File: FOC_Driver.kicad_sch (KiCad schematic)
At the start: 0 parts

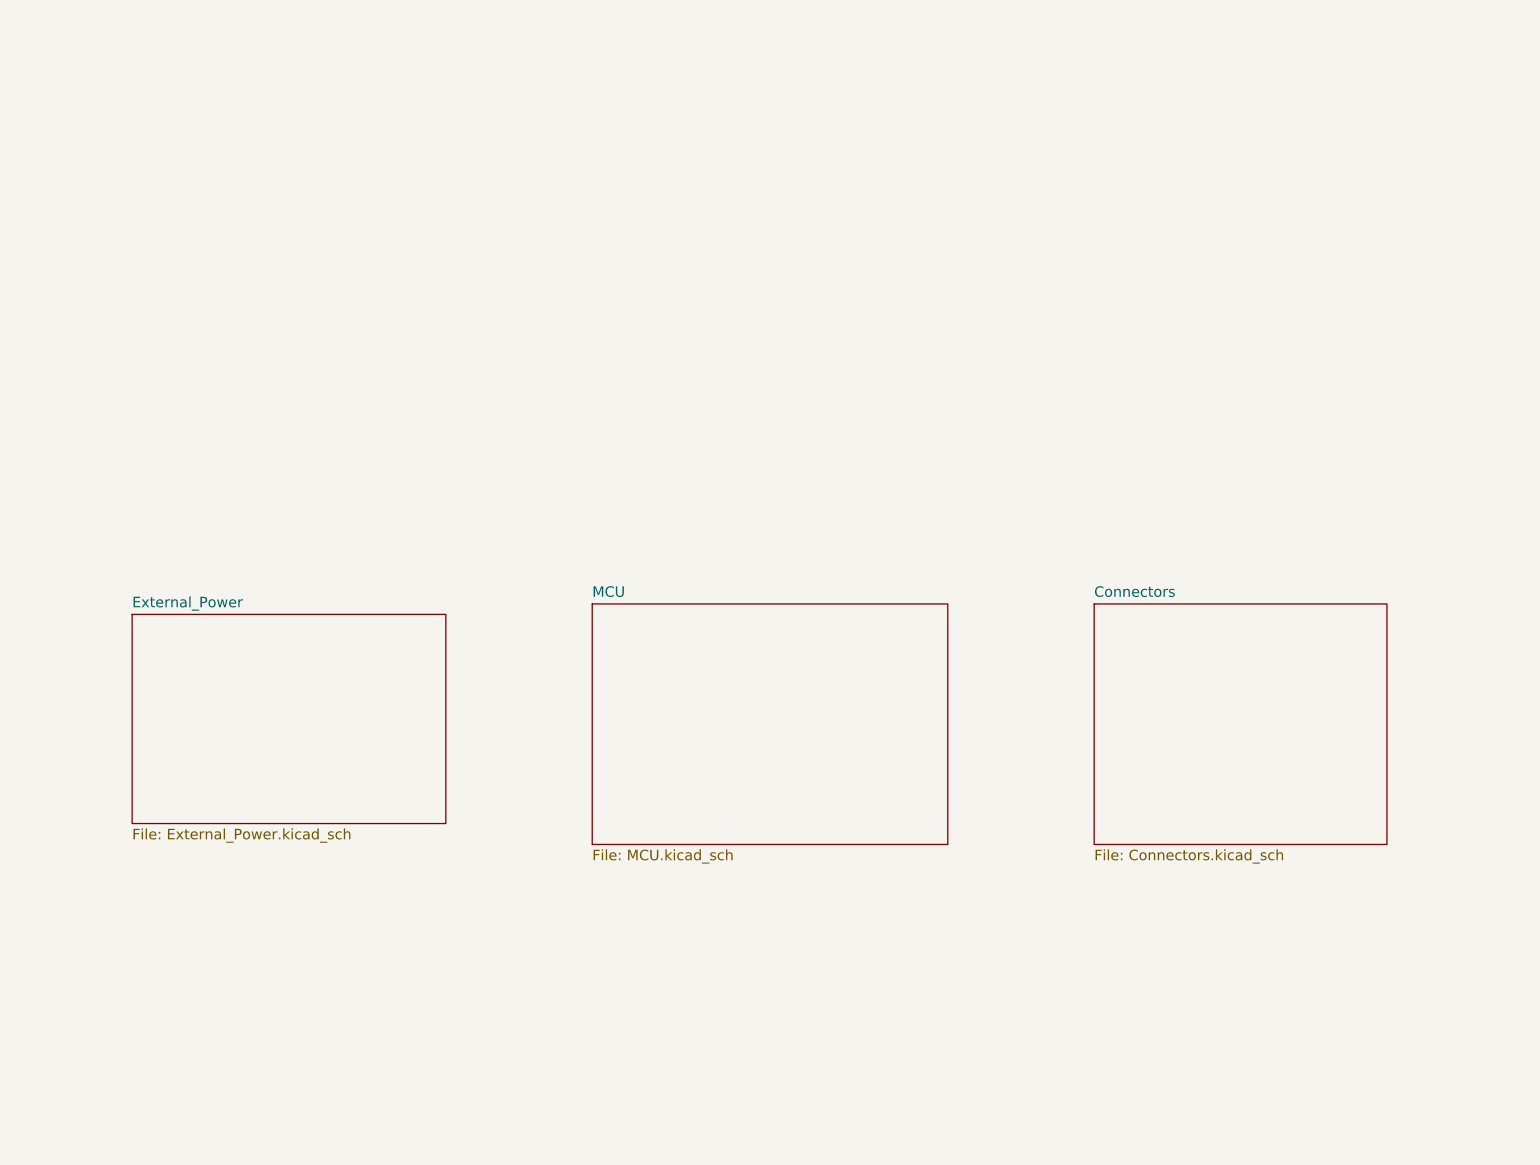
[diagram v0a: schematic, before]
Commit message: Wip
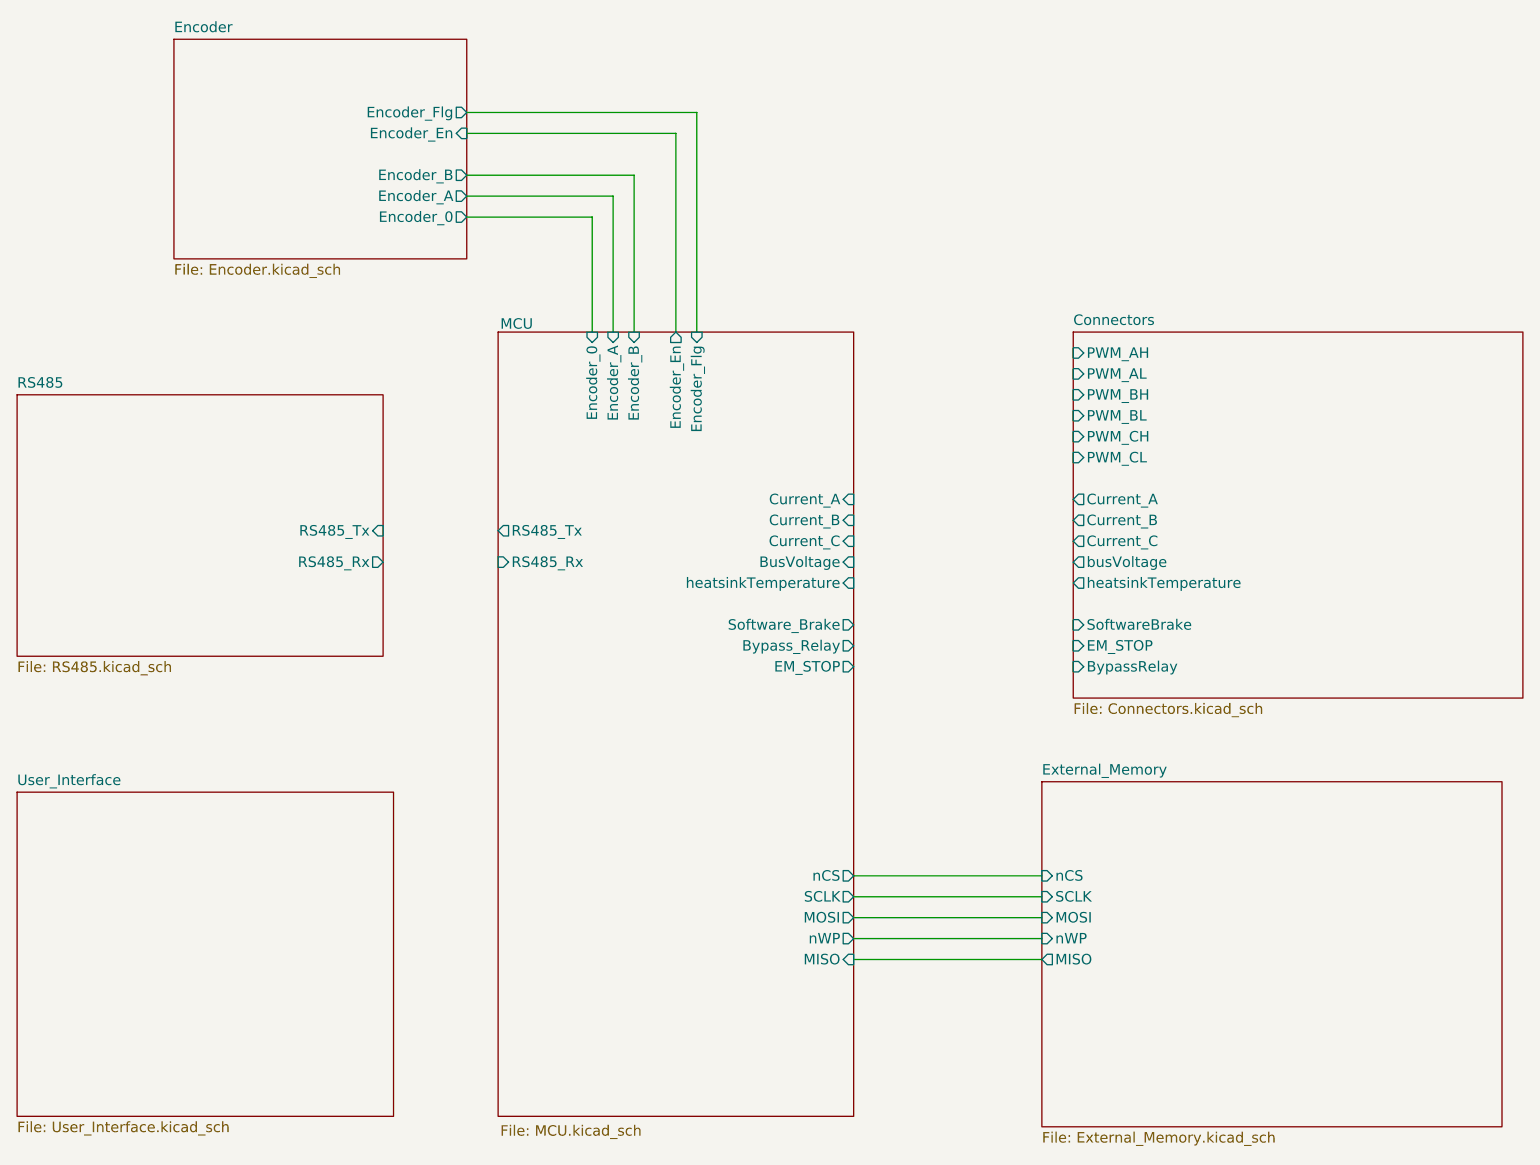
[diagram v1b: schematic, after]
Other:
- removed sheet External_Power
- added sheet Encoder (Encoder.kicad_sch)
- added sheet External_Memory (External_Memory.kicad_sch)
- added sheet RS485 (RS485.kicad_sch)
- added sheet User_Interface (User_Interface.kicad_sch)
- sheet Connectors ports: added BypassRelay, Current_A, Current_B, Current_C, EM_STOP, PWM_AH, PWM_AL, PWM_BH, PWM_BL, PWM_CH, PWM_CL, SoftwareBrake, busVoltage, heatsinkTemperature; removed none
- sheet MCU ports: added BusVoltage, Bypass_Relay, Current_A, Current_B, Current_C, EM_STOP, Encoder_0, Encoder_A, Encoder_B, Encoder_En, Encoder_Flg, MISO, MOSI, RS485_Rx, RS485_Tx, SCLK, Software_Brake, heatsinkTemperature, nCS, nWP; removed none
